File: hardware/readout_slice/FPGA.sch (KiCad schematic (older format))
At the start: 9 parts

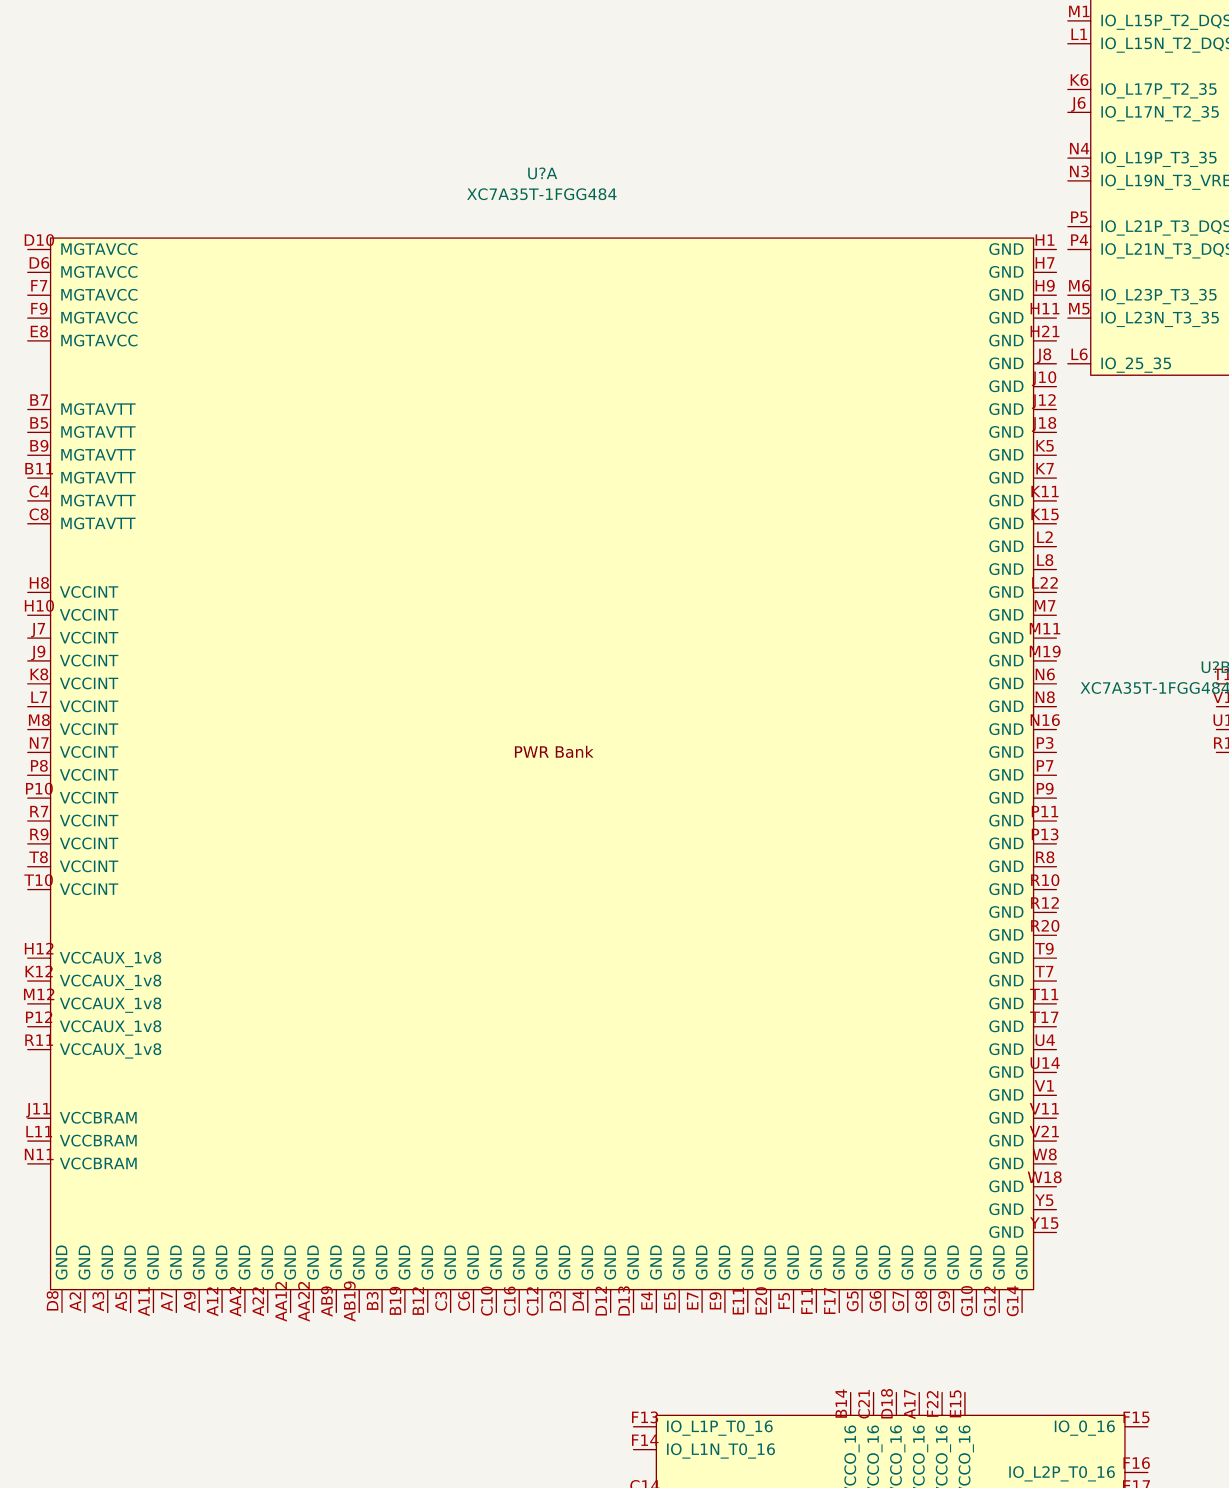
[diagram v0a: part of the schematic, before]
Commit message: more work on readout_slice
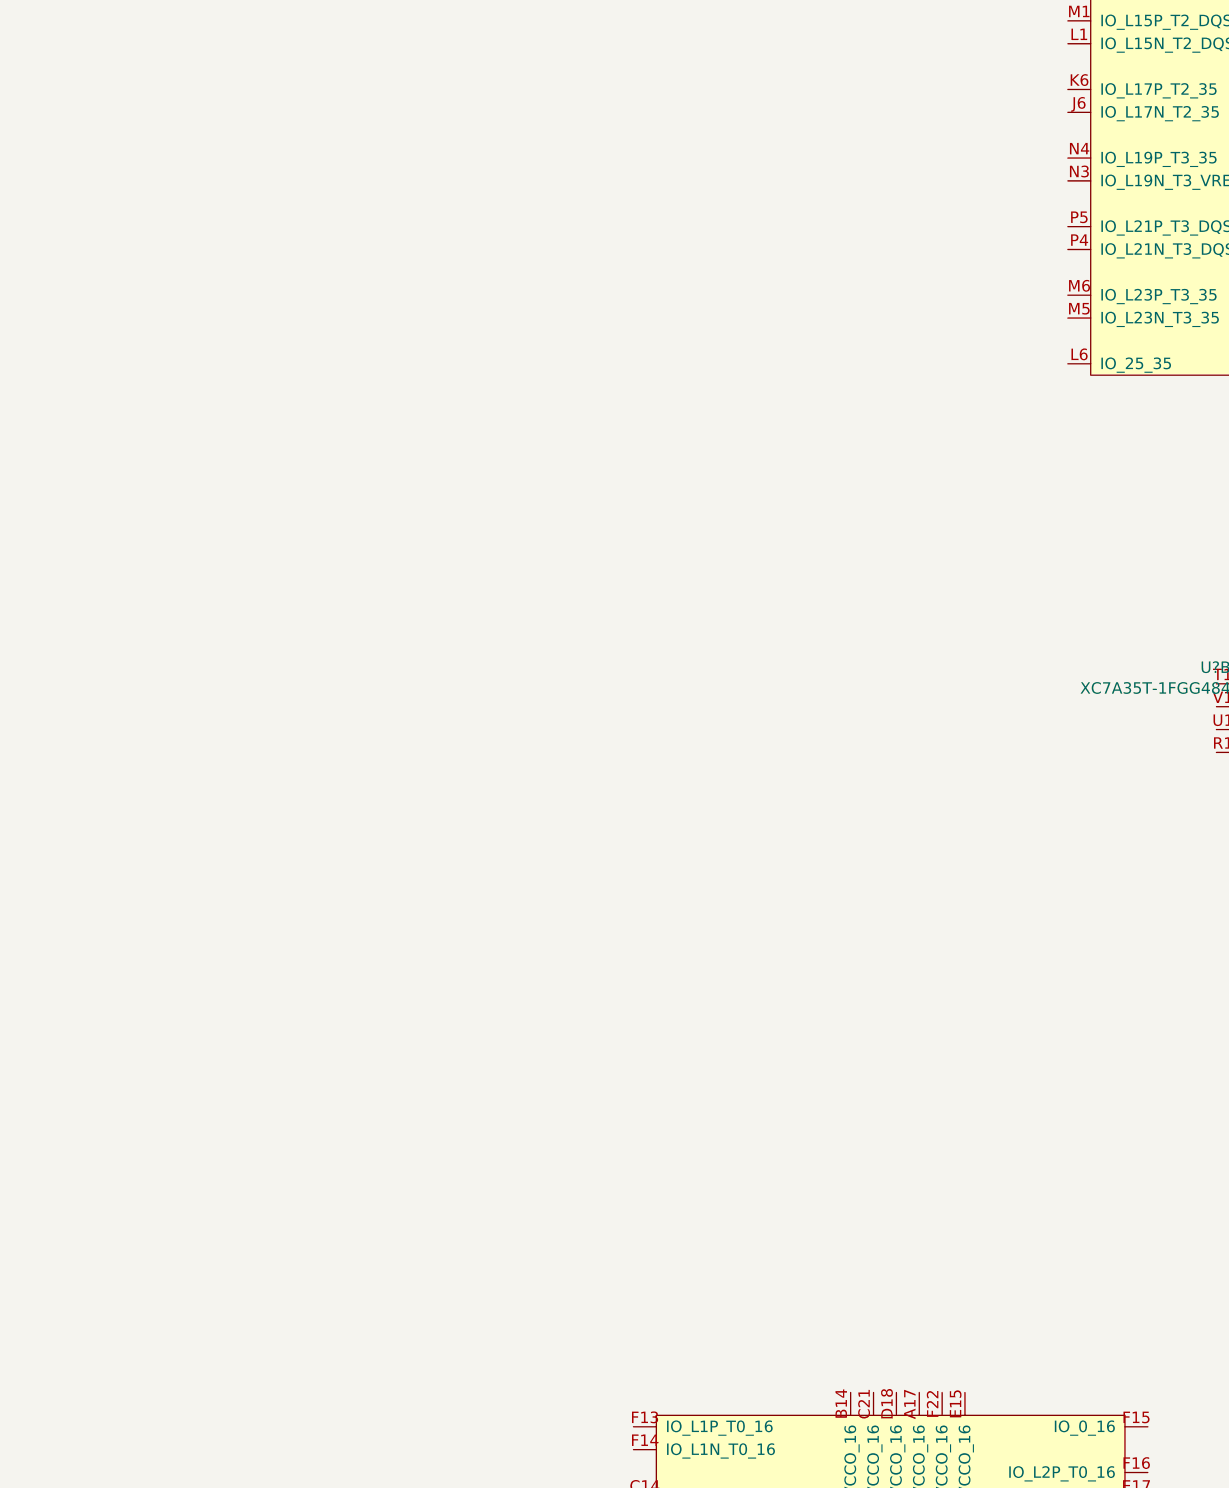
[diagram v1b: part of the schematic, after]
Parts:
- removed U?: XC7A35T-1FGG484, symbol readout:XC7A35T-1FGG484
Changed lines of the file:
@@
-$Comp
-L readout:XC7A35T-1FGG484 U?
-U 1 1 604A9F40
-P 650 150
-F 0 "U?" H 500 431 50  0000 C CNN
-F 1 "XC7A35T-1FGG484" H 500 340 50  0000 C CNN
-F 2 "" H -450 300 50  0001 C CNN
-F 3 "" H -450 300 50  0001 C CNN
-	1    650  150
-	1    0    0    -1
-$EndComp
 $Comp
 L readout:XC7A35T-1FGG484 U?

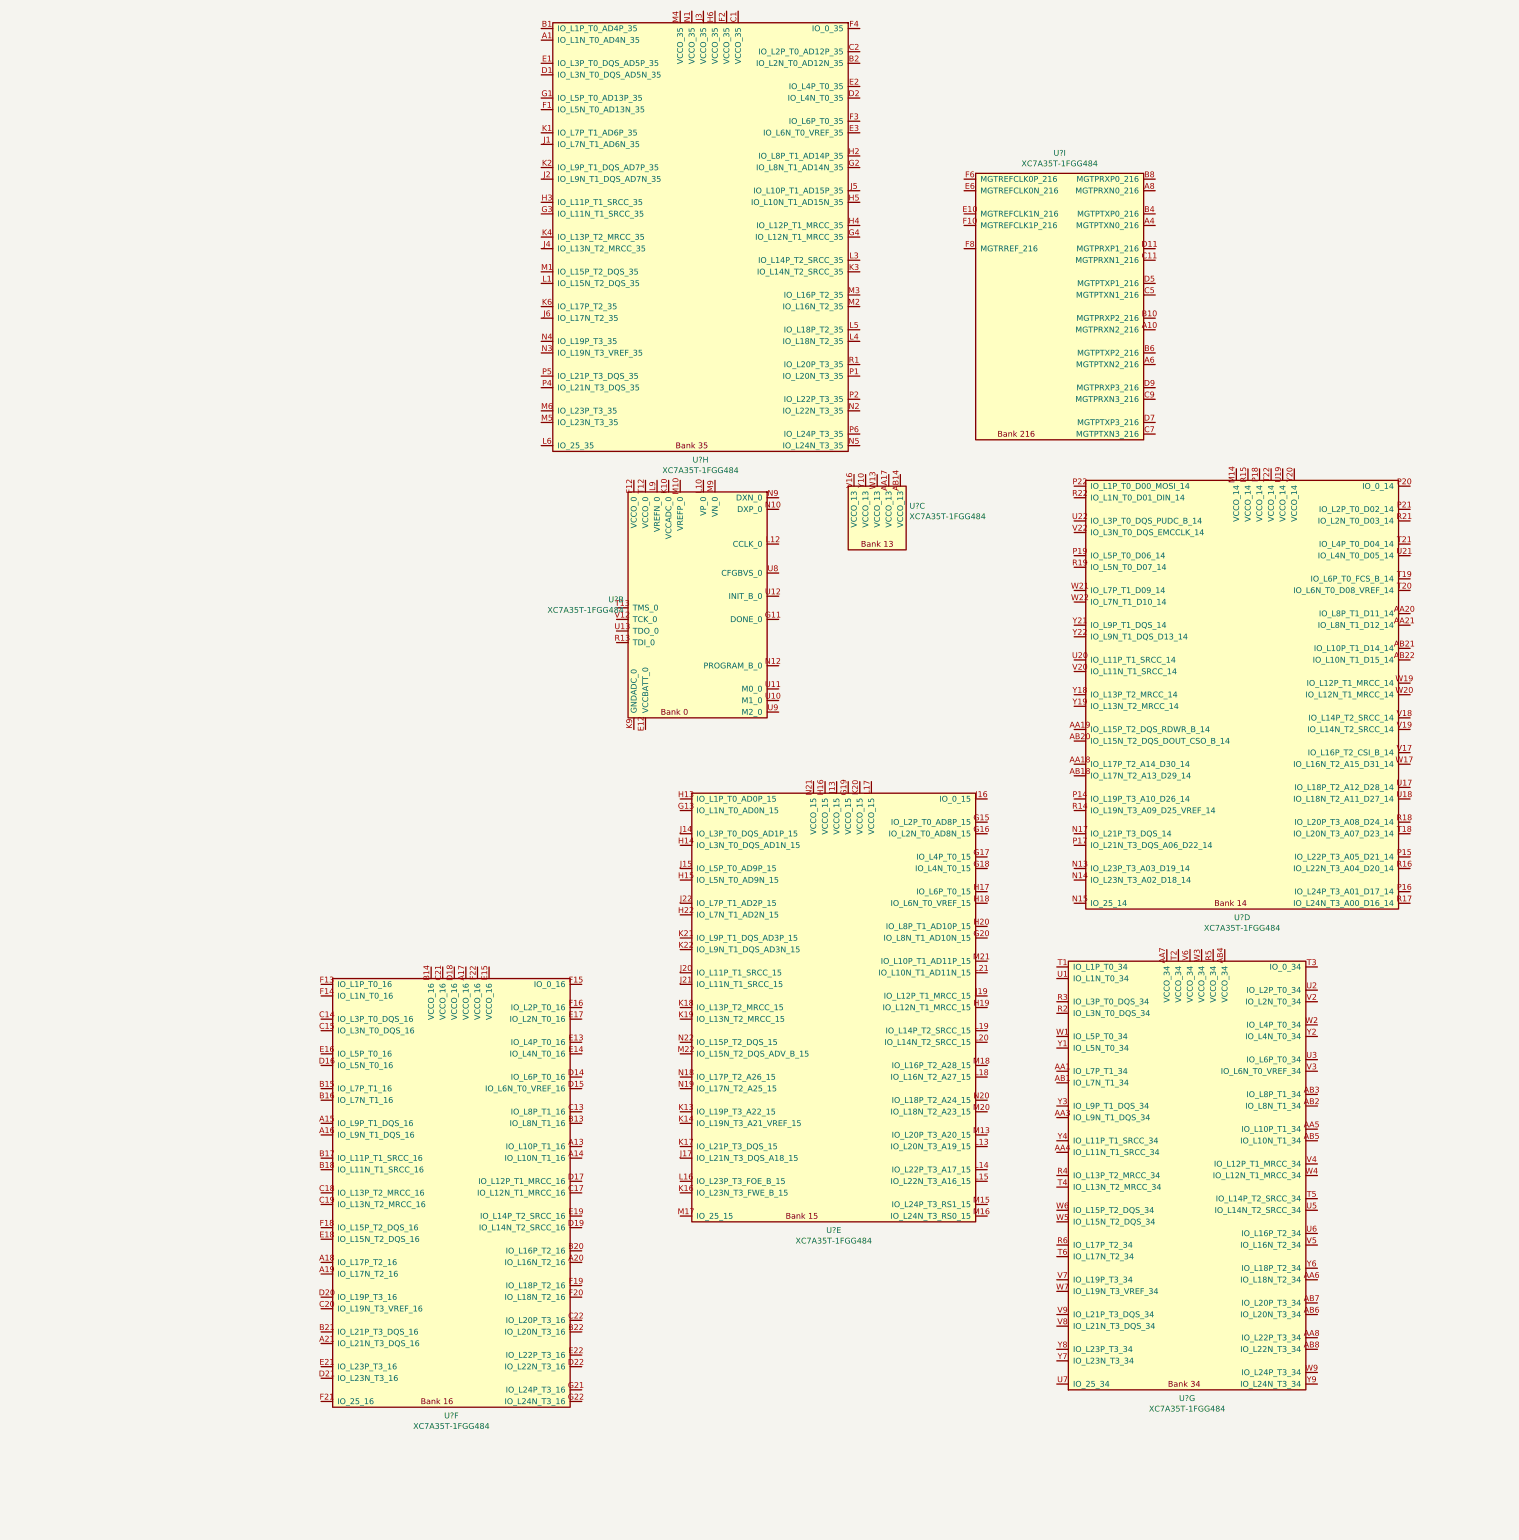
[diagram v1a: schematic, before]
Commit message: working more on readout_slice schematic
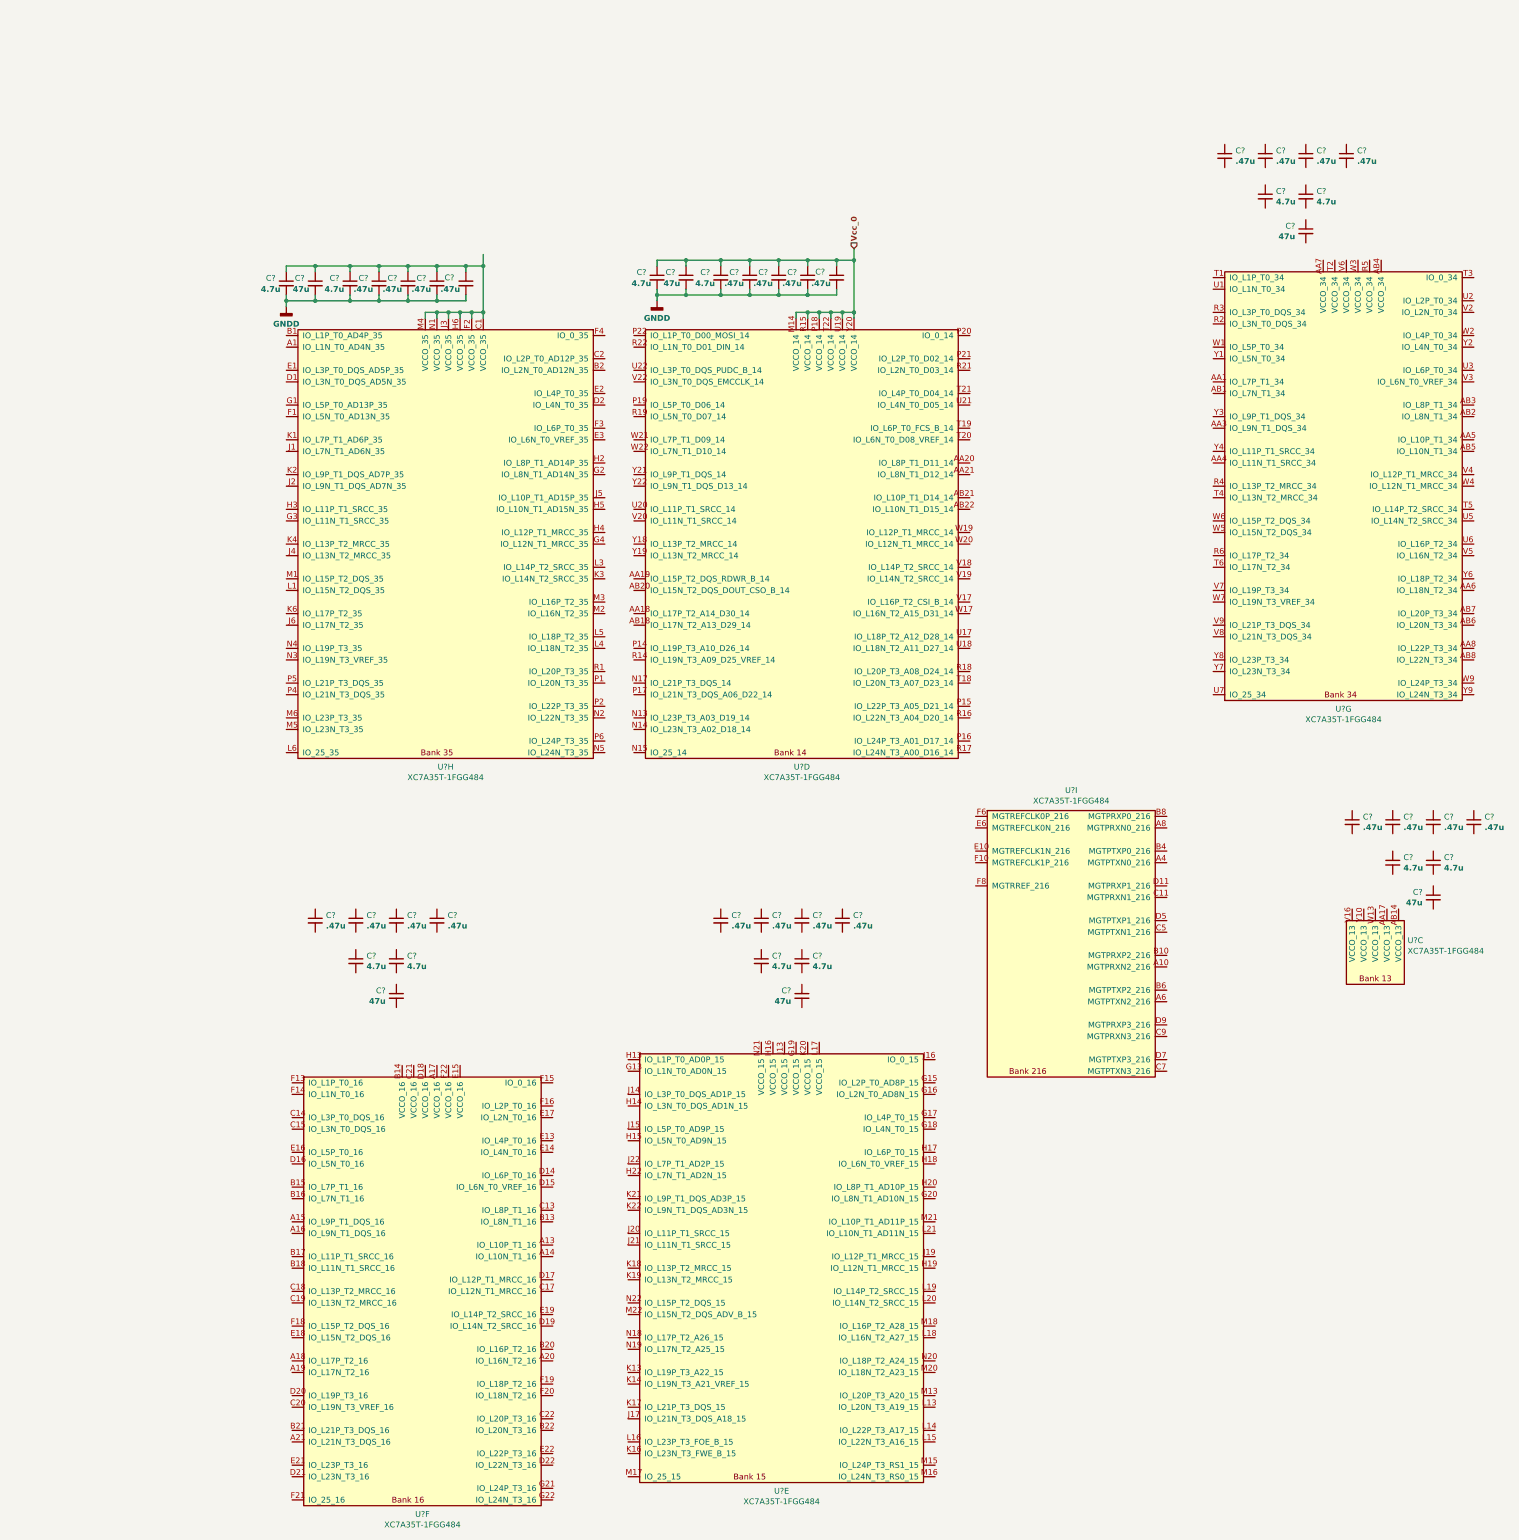
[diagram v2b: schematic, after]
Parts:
- removed U?: XC7A35T-1FGG484, symbol readout:XC7A35T-1FGG484
- added C? (x6): 47u, symbol Device:C_Small
- added C? (x12): 4.7u, symbol Device:C_Small
- added C? (x24): .47u, symbol Device:C_Small
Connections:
- net Vcc_0: now reaches U?.M14 (VCCO_14)
- net Vcc_0: now also U?.P18 (VCCO_14), U?.R15 (VCCO_14), U?.T22 (VCCO_14), U?.U19 (VCCO_14), U?.Y20 (VCCO_14), C?.1, C?.1, C?.1, C?.1, C?.1, C?.1, C?.1
- net at U?.C1 (VCCO_35): now also U?.F2 (VCCO_35), U?.H6 (VCCO_35), U?.J3 (VCCO_35), U?.M4 (VCCO_35), U?.N1 (VCCO_35), C?.1, C?.1, C?.1, C?.1, C?.1, C?.1, C?.1
- new net GNDD: C?.2, C?.2, C?.2, C?.2, C?.2, C?.2, C?.2, C?.2, C?.2, C?.2, C?.2, C?.2, C?.2, C?.2
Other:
- moved on the sheet: U?C, U?D, U?E, U?F, U?G, U?H, U?I
